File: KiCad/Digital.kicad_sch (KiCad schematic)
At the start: 39 parts, among them IC1 PIC24H, J2 DE9_Plug_MountingHoles, J3 DE9_Plug_MountingHoles, J4 Conn_01x03, J7 Conn_01x05, SW1 SW_DP3T, SW2 SW_DP3T, SW3 SW_DP3T, SW4 OP/CL, SW7 OP/CL, U2 MCP2551-I-SN, U3 PCF8574P, Y1 Crystal

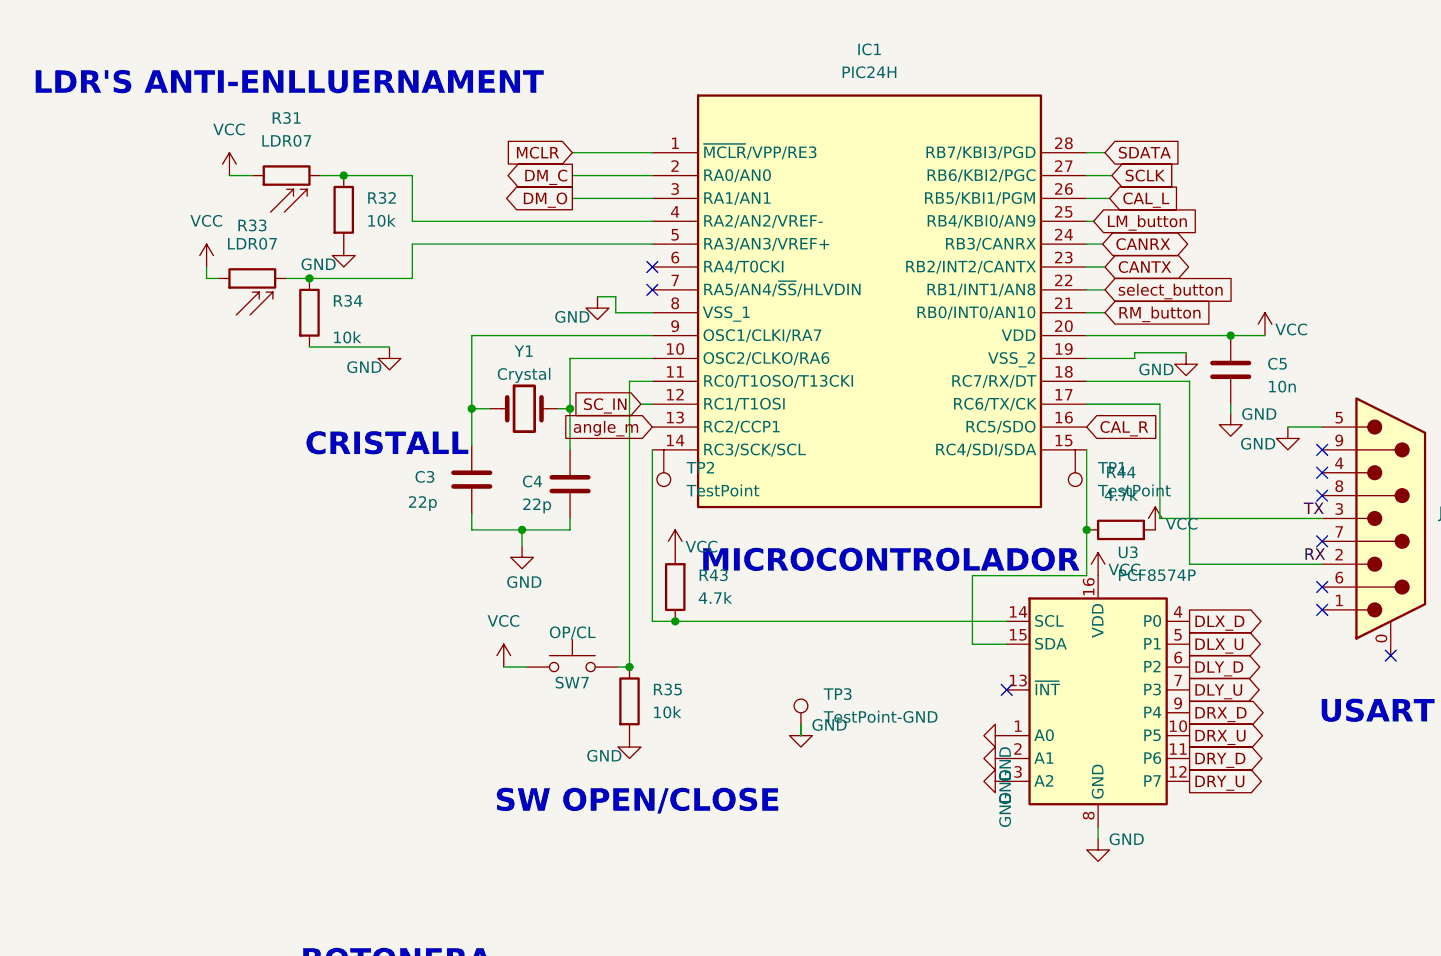
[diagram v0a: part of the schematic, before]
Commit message: correcions de pcb
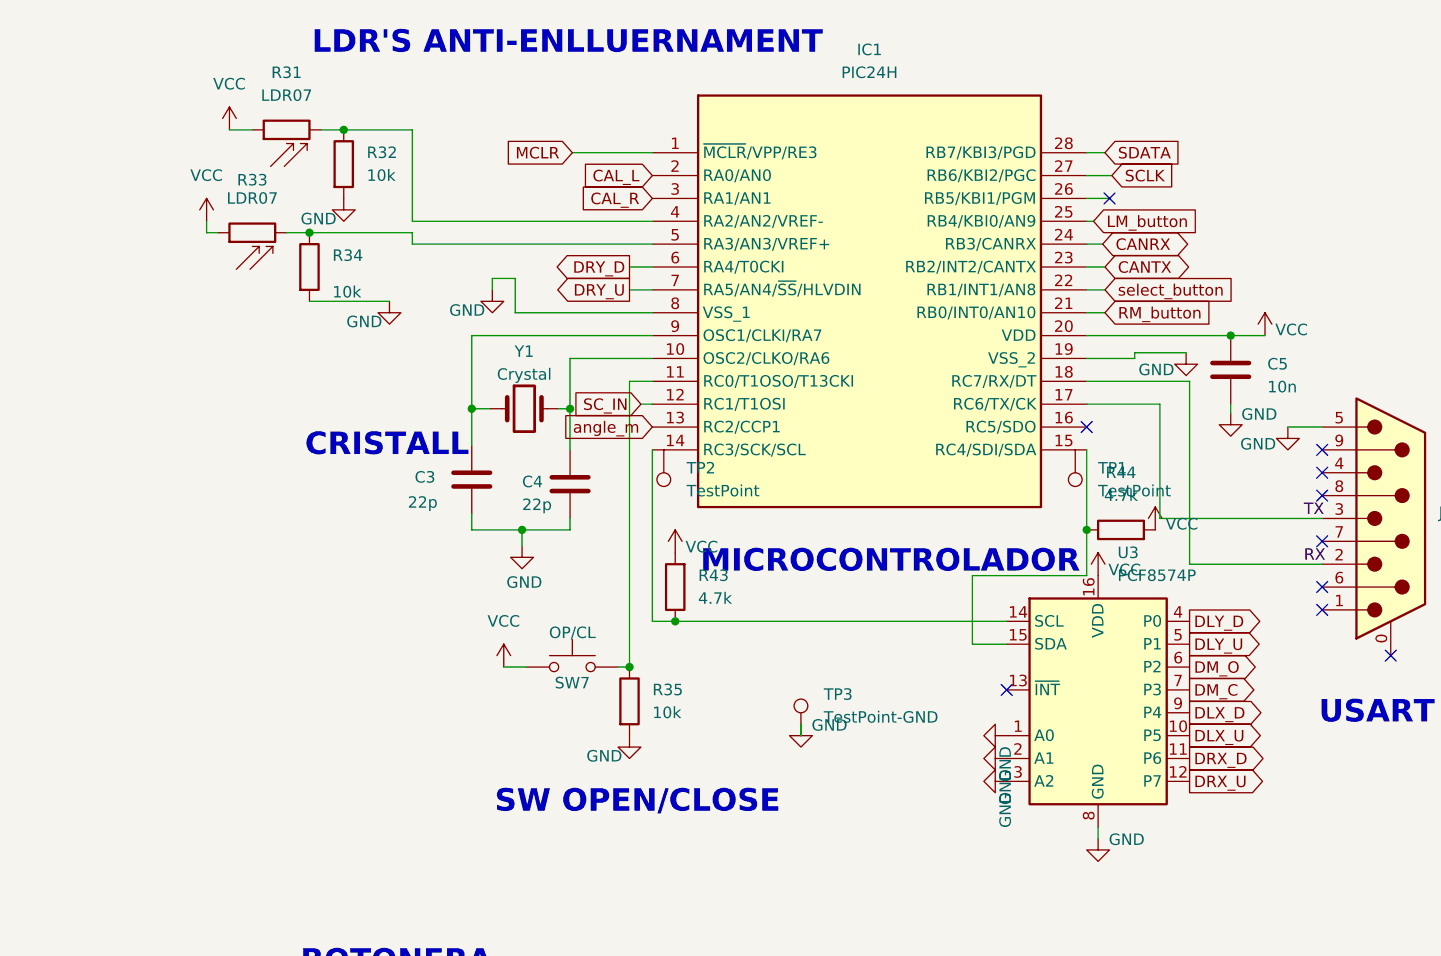
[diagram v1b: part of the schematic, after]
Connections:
- net CAL_L: now also IC1.2 (RA0/AN0); no longer IC1.26 (RB5/KBI1/PGM)
- net CAL_R: now also IC1.3 (RA1/AN1); no longer IC1.16 (RC5/SDO)
- net DLX_D: now also U3.9 (P4); no longer U3.4 (P0)
- net DLX_U: now also U3.10 (P5); no longer U3.5 (P1)
- net DLY_D: now also U3.4 (P0); no longer U3.6 (P2)
- net DLY_U: now also U3.5 (P1); no longer U3.7 (P3)
- net DM_C: now also U3.7 (P3); no longer IC1.2 (RA0/AN0)
- net DM_O: now also U3.6 (P2); no longer IC1.3 (RA1/AN1)
- net DRX_D: now also U3.11 (P6); no longer U3.9 (P4)
- net DRX_U: now also U3.12 (P7); no longer U3.10 (P5)
- net DRY_D: now also IC1.6 (RA4/T0CKI); no longer U3.11 (P6)
- net DRY_U: now also IC1.7 (RA5/AN4/~{SS}/HLVDIN); no longer U3.12 (P7)
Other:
- moved on the sheet: R31, R32, R33, R34

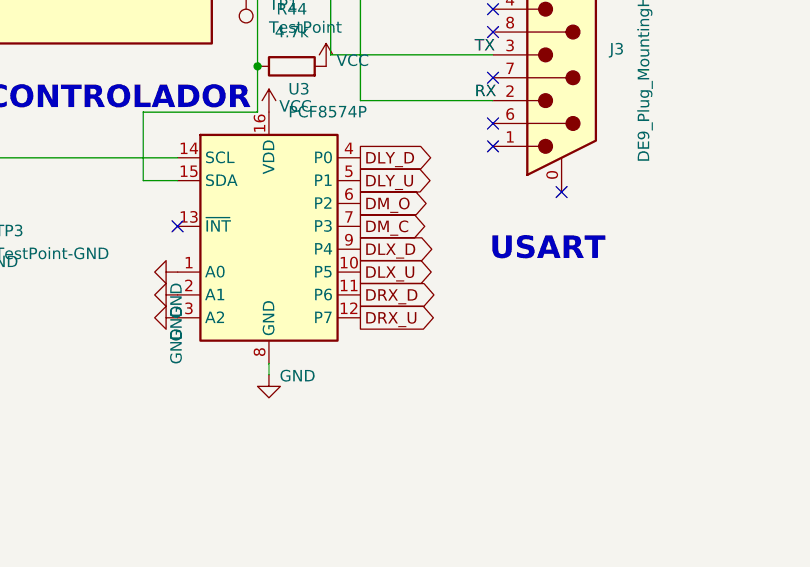
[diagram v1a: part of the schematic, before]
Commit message: pcb Tota connectada
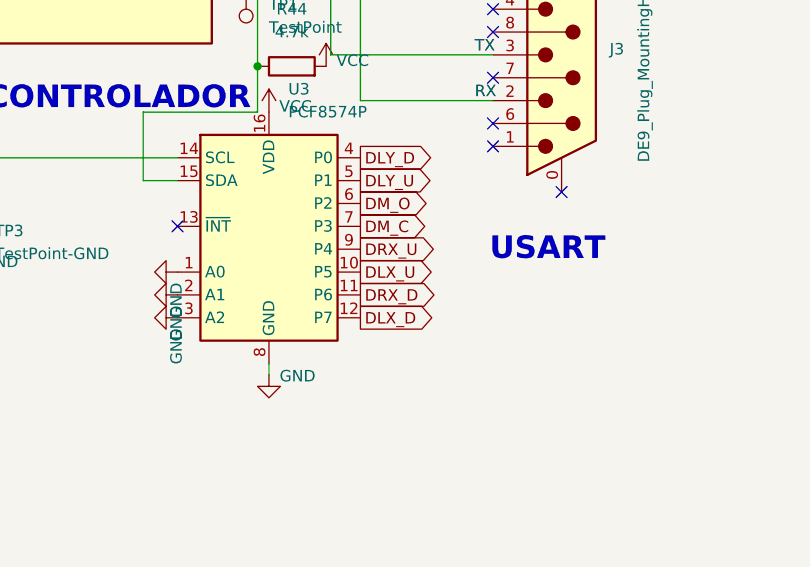
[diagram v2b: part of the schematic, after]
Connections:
- net DLX_D: now also U3.12 (P7); no longer U3.9 (P4)
- net DRX_U: now also U3.9 (P4); no longer U3.12 (P7)
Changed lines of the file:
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@@
+		)
+	)
+	(global_label "DRX_U"
+		(shape output)
+		(at 143.51 90.17 0)
+		(fields_autoplaced yes)
+		(effects
+			(font
+				(size 1.27 1.27)
+			)
+			(justify left)
+		)
+		(property "Intersheetrefs" "${INTERSHEET_REFS}"
+			(at 152.5428 90.17 0)
+			(effects
+				(font
+					(size 1.27 1.27)
+				)
+				(justify left)
+				(hide yes)
+			)
 		)
 	)
@@
 		)
 	)
+	(global_label "DLX_D"
+		(shape output)
+		(at 143.51 97.79 0)
+		(fields_autoplaced yes)
+		(effects
+			(font
+				(size 1.27 1.27)
+			)
+			(justify left)
+		)
+		(property "Intersheetrefs" "${INTERSHEET_REFS}"
+			(at 152.2404 97.79 0)
+			(effects
+				(font
+					(size 1.27 1.27)
+				)
+				(justify left)
+				(hide yes)
+			)
+		)
+	)
 	(global_label "CAL_L"
 		(shape input)
@@
 		)
 	)
-	(global_label "DLX_D"
-		(shape output)
-		(at 143.51 90.17 0)
-		(fields_autoplaced yes)
-		(effects
-			(font
-				(size 1.27 1.27)
-			)
-			(justify left)
-		)
-		(property "Intersheetrefs" "${INTERSHEET_REFS}"
-			(at 152.2404 90.17 0)
-			(effects
-				(font
-					(size 1.27 1.27)
-				)
-				(justify left)
-				(hide yes)
-			)
-		)
-	)
 	(global_label "DRY_D"
 		(shape output)
@@
 			(effects
 				(font
-					(size 1.27 1.27)
-				)
-				(justify left)
-				(hide yes)
-			)
-		)
-	)
-	(global_label "DRX_U"
-		(shape output)
-		(at 143.51 97.79 0)
-		(fields_autoplaced yes)
-		(effects
-			(font
-				(size 1.27 1.27)
-			)
-			(justify left)
-		)
-		(property "Intersheetrefs" "${INTERSHEET_REFS}"
-			(at 152.5428 97.79 0)
-			(effects
-				(font
